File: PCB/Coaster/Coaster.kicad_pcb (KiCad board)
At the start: 2 copper layers, 202 x 100 mm, 84 parts, among them J1 Join, J2 Shelly, J3 USB-C, P1 TestPoint, P10 TestPoint, P11 TestPoint, P12 TestPoint, P13 TestPoint, P14 TestPoint, P15 TestPoint, P16 TestPoint, P17 TestPoint, P2 TestPoint, P5 TestPoint, P6 TestPoint, P7 TestPoint, P8 TestPoint, P9 TestPoint, T1 TestPoint, T10 TestPoint, T11 TestPoint, T12 TestPoint, T13 TestPoint, T14 TestPoint, T15 TestPoint, T16 TestPoint, T17 TestPoint, T2 TestPoint, T5 TestPoint, T6 TestPoint, T7 TestPoint, T8 TestPoint, T9 TestPoint, U1 ESP32-PICO-MINI-02, U2 LMR16006XDDCR, U3 QR

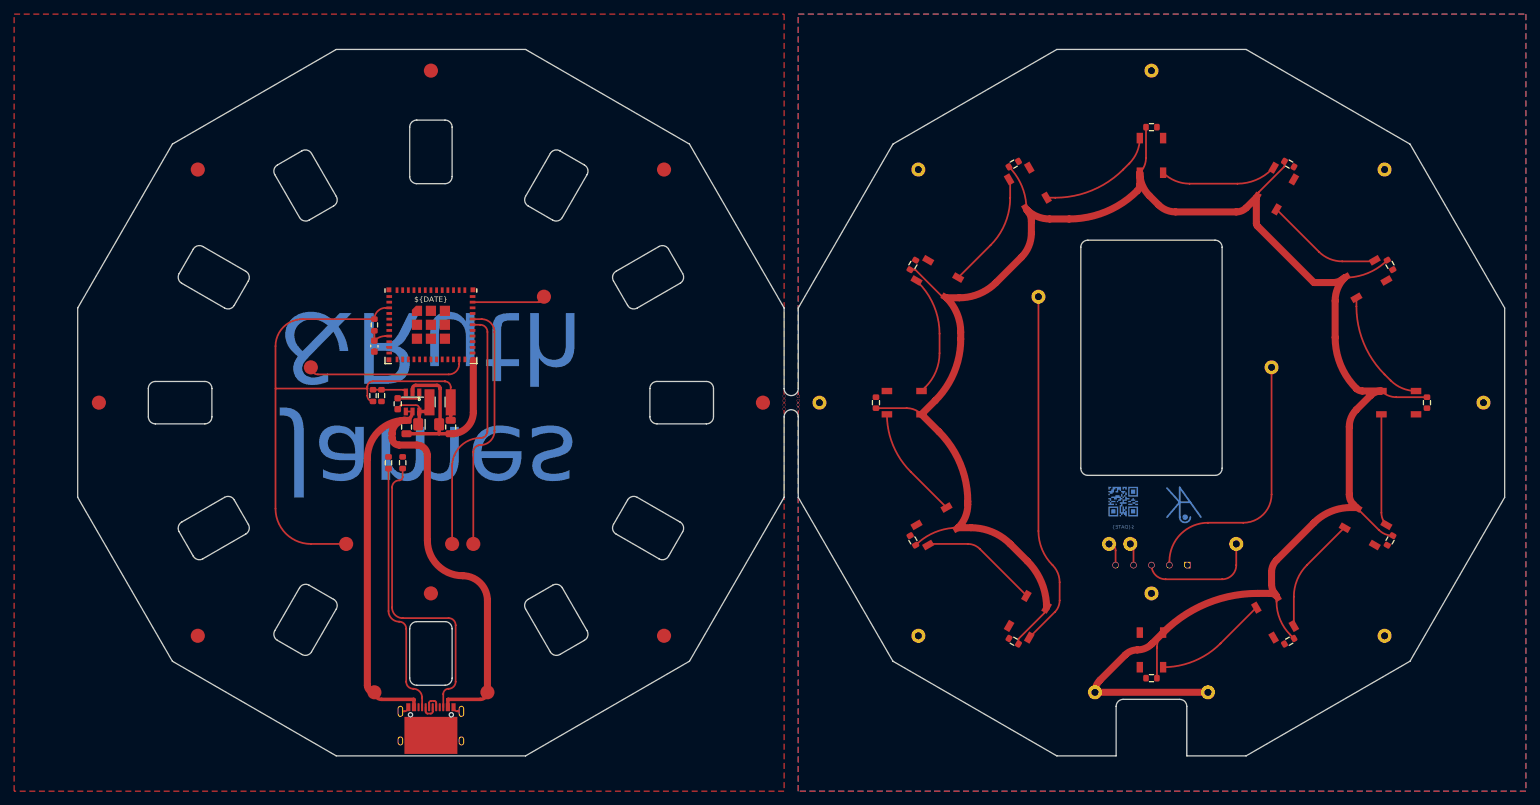
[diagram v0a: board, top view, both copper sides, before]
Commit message: Much tidying
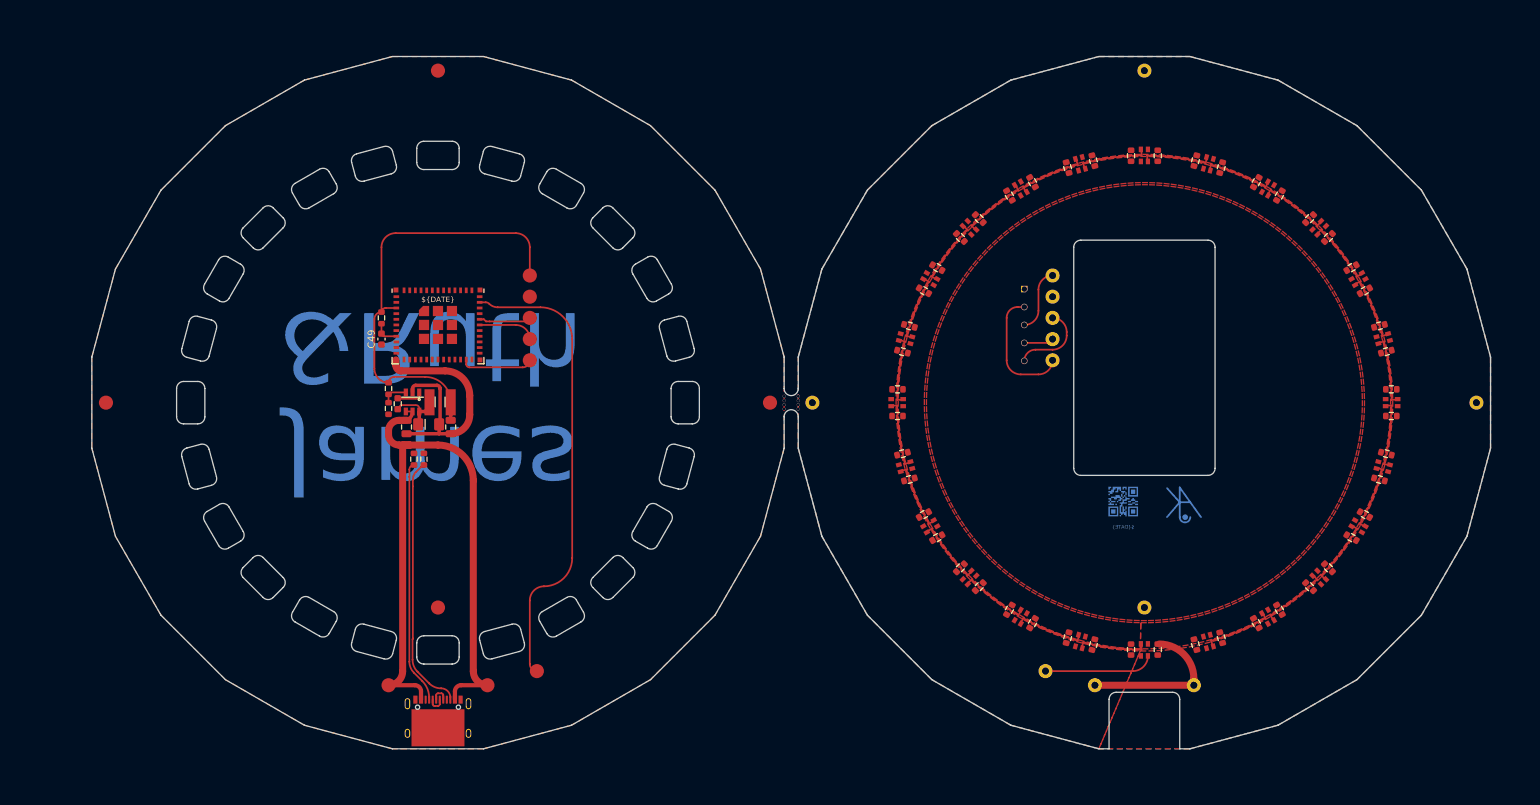
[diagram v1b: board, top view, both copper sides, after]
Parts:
- removed P13, P14, P15, P16, P17: TestPoint, RevK:PAD
- removed R6: 5K1, RevK:R_0603
- removed R7: 100k 1%, RevK:R_0603
- removed R8: 30k 1%, RevK:R_0603
- removed T13, T14, T15, T16, T17: TestPoint, RevK:PAD-LINK
- added C17: 10nF, RevK:C_0603, F.Cu at (229.3, 80.9)
- added C18: 10nF, RevK:C_0603, F.Cu at (233.3, 89.1)
- added C19: 10nF, RevK:C_0603, F.Cu at (234.9, 98.1)
- added C20: 10nF, RevK:C_0603, F.Cu at (234.2, 107.2)
- added C21: 10nF, RevK:C_0603, F.Cu at (231.2, 115.8)
- added C22: 10nF, RevK:C_0603, F.Cu at (226.1, 123.4)
- added C23: 10nF, RevK:C_0603, F.Cu at (219.1, 129.3)
- added C24: 10nF, RevK:C_0603, F.Cu at (210.9, 133.3)
- added C25: 10nF, RevK:C_0603, F.Cu at (198.1, 134.9)
- added C26: 10nF, RevK:C_0603, F.Cu at (189.1, 133.3)
- added C27: 10nF, RevK:C_0603, F.Cu at (180.9, 129.3)
- added C28: 10nF, RevK:C_0603, F.Cu at (173.9, 123.4)
- added C29: 10nF, RevK:C_0603, F.Cu at (168.8, 115.8)
- added C30: 10nF, RevK:C_0603, F.Cu at (165.8, 107.2)
- added C31: 10nF, RevK:C_0603, F.Cu at (165.1, 98.1)
- added C32: 10nF, RevK:C_0603, F.Cu at (166.7, 89.1)
- added C33: 10nF, RevK:C_0603, F.Cu at (170.7, 80.9)
- added C34: 10nF, RevK:C_0603, F.Cu at (176.6, 74.0)
- added C35: 10nF, RevK:C_0603, F.Cu at (184.2, 68.8)
- added C36: 10nF, RevK:C_0603, F.Cu at (192.8, 65.8)
- added C37: 10nF, RevK:C_0603, F.Cu at (201.9, 65.0)
- added C38: 10nF, RevK:C_0603, F.Cu at (210.9, 66.7)
- added C39: 10nF, RevK:C_0603, F.Cu at (219.1, 70.7)
- added C40: 10nF, RevK:C_0603, F.Cu at (226.1, 76.6)
- added C41: 10nF, RevK:C_0603, F.Cu at (231.2, 84.2)
- added C42: 10nF, RevK:C_0603, F.Cu at (234.2, 92.8)
- added C43: 10nF, RevK:C_0603, F.Cu at (234.9, 101.9)
- added C44: 10nF, RevK:C_0603, F.Cu at (233.3, 110.9)
- added C45: 10nF, RevK:C_0603, F.Cu at (229.3, 119.1)
- added C46: 10nF, RevK:C_0603, F.Cu at (223.4, 126.0)
- added C47: 10nF, RevK:C_0603, F.Cu at (215.8, 131.2)
- added C48: 10nF, RevK:C_0603, F.Cu at (207.2, 134.2)
- added C49: 10nF, Capacitor_SMD:C_0603_1608Metric, F.Cu at (92.0, 91.0)
- added C50: 100nF, RevK:C_0603_, F.Cu at (94.3, 100.2)
- added C51: 2.2uF, RevK:C_0805_, F.Cu at (95.5, 103.5)
- added C52: 10uF, RevK:C_0805_, F.Cu at (101.8, 103.5)
- added D13: WS2818B, RevK:SMD2020, F.Cu at (200.0, 65.0)
- added D15: WS2818B, RevK:SMD2020, F.Cu at (217.5, 69.7)
- added D16: WS2818B, RevK:SMD2020, F.Cu at (224.8, 75.2)
- added D17: WS2818B, RevK:SMD2020, F.Cu at (230.3, 82.5)
- added D18: WS2818B, RevK:SMD2020, F.Cu at (233.8, 90.9)
- added D19: WS2818B, RevK:SMD2020, F.Cu at (235.0, 100.0)
- added D20: WS2818B, RevK:SMD2020, F.Cu at (233.8, 109.1)
- added D21: WS2818B, RevK:SMD2020, F.Cu at (230.3, 117.5)
- added D22: WS2818B, RevK:SMD2020, F.Cu at (224.8, 124.8)
- added D23: WS2818B, RevK:SMD2020, F.Cu at (217.5, 130.3)
- added D24: WS2818B, RevK:SMD2020, F.Cu at (209.1, 133.8)
- added D25: Schottky, RevK:D_1206_, F.Cu at (98.7, 103.1)
- added H13: MountingHole, RevK:LEDHOLE, F.Cu at (100.0, 65.0)
- added H14: MountingHole, RevK:LEDHOLE, F.Cu at (109.1, 66.2)
- added H15: MountingHole, RevK:LEDHOLE, F.Cu at (117.5, 69.7)
- added H16: MountingHole, RevK:LEDHOLE, F.Cu at (124.8, 75.2)
- added H17: MountingHole, RevK:LEDHOLE, F.Cu at (130.3, 82.5)
- added H18: MountingHole, RevK:LEDHOLE, F.Cu at (133.8, 90.9)
- added H19: MountingHole, RevK:LEDHOLE, F.Cu at (135.0, 100.0)
- added H20: MountingHole, RevK:LEDHOLE, F.Cu at (133.8, 109.1)
- added H21: MountingHole, RevK:LEDHOLE, F.Cu at (130.3, 117.5)
- added H22: MountingHole, RevK:LEDHOLE, F.Cu at (124.8, 124.8)
- added H23: MountingHole, RevK:LEDHOLE, F.Cu at (117.5, 130.3)
- added H24: MountingHole, RevK:LEDHOLE, F.Cu at (109.1, 133.8)
- added P3: TestPoint, RevK:PAD, F.Cu at (113.0, 88.0)
- added P4: TestPoint, RevK:PAD, F.Cu at (113.0, 91.0)
- added R2: 5K1, RevK:R_0603, F.Cu at (96.6, 108.0)
- added R3: 5K1, RevK:R_0603, F.Cu at (98.0, 108.0)
- added R4: 100k 1%, RevK:R_0603, F.Cu at (93.0, 98.0)
- added T3: TestPoint, RevK:PAD-LINK, F.Cu at (187.0, 88.0)
- added T4: TestPoint, RevK:PAD-LINK, F.Cu at (187.0, 91.0)
- C13: value 100nF -> 10nF; footprint RevK:C_0603_ -> RevK:C_0603
- C14: value 2.2uF -> 10nF; footprint RevK:C_0805_ -> RevK:C_0603
- C15: value 10uF -> 10nF; footprint RevK:C_0805_ -> RevK:C_0603
- C16: footprint Capacitor_SMD:C_0603_1608Metric -> RevK:C_0603
- D1, D10, D11, D12, D2, D3, D4, D5, D6, D7, D8, D9: footprint RevK:SMD5050 -> RevK:SMD2020
- D14: value Schottky -> WS2818B; footprint RevK:D_1206_ -> RevK:SMD2020
- J1: value Join -> USB-C; footprint RevK:PCB-Join -> RevK:USC16-TR
- J3: value USB-C -> Join; footprint RevK:USC16-TR -> RevK:PCB-Join
- R5: value 5K1 -> 30k 1%
- moved C16 133.6 mm to (223.4, 74.0), turned to 45 degrees
- moved C15 119.2 mm to (215.8, 68.8), turned to 60 degrees
- moved C14 117.9 mm to (207.2, 65.8), turned to 75 degrees
- moved D14 116.4 mm to (209.1, 66.2), turned to 75 degrees
- moved C13 109.6 mm to (198.1, 65.0), turned to 90 degrees
- moved P7 86.3 mm to (114.0, 138.0)
- moved T7 86.3 mm to (186.0, 138.0)
- moved C5 74.8 mm to (170.7, 119.1), turned to -150 degrees
- moved P8 74.0 mm to (100.0, 53.0)
- moved T8 74.0 mm to (200.0, 53.0)
- moved D5 70.9 mm to (169.7, 117.5), turned to -150 degrees
- moved C6 69.9 mm to (166.7, 110.9), turned to -165 degrees
- moved H5 69.1 mm to (69.7, 117.5), turned to 120 degrees
- moved C4 68.5 mm to (176.6, 126.0), turned to -135 degrees
- moved J3 68.4 mm to (150.0, 100.0)
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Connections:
- C16 pad 1: GND -> VCC
- C16 pad 2: Net-(C16-Pad2) -> GND2
- D1 pad 2: unconnected-(D1-Pad2) -> Net-(D1-Pad2)
- D1 pad 4: Net-(D1-Pad4) -> LED
- D11 pad 2: Net-(D10-Pad4) -> Net-(D11-Pad2)
- D11 pad 4: Net-(D11-Pad4) -> Net-(D10-Pad2)
- D12 pad 2: Net-(D11-Pad4) -> Net-(D12-Pad2)
- D12 pad 4: LED -> Net-(D11-Pad2)
- D2 pad 2: Net-(D1-Pad4) -> Net-(D2-Pad2)
- D2 pad 4: Net-(D2-Pad4) -> Net-(D1-Pad2)
- D3 pad 2: Net-(D2-Pad4) -> Net-(D3-Pad2)
- D3 pad 4: Net-(D3-Pad4) -> Net-(D2-Pad2)
- D4 pad 2: Net-(D3-Pad4) -> Net-(D4-Pad2)
- D4 pad 4: Net-(D4-Pad4) -> Net-(D3-Pad2)
- D5 pad 2: Net-(D4-Pad4) -> Net-(D5-Pad2)
- D5 pad 4: Net-(D5-Pad4) -> Net-(D4-Pad2)
- D6 pad 2: Net-(D5-Pad4) -> Net-(D6-Pad2)
- D6 pad 4: Net-(D6-Pad4) -> Net-(D5-Pad2)
- D7 pad 2: Net-(D6-Pad4) -> Net-(D7-Pad2)
- D7 pad 4: Net-(D7-Pad4) -> Net-(D6-Pad2)
- D8 pad 2: Net-(D7-Pad4) -> Net-(D8-Pad2)
- D8 pad 4: Net-(D8-Pad4) -> Net-(D7-Pad2)
- D9 pad 2: Net-(D8-Pad4) -> Net-(D10-Pad4)
- D9 pad 4: Net-(D10-Pad2) -> Net-(D8-Pad2)
- P10 pad 1: Net-(P10-Pad1) -> GND
- P11 pad 1: +3V3 -> GND
- P12 pad 1: Net-(P12-Pad1) -> GND
- P5 pad 1: GND -> +3V3
- P6 pad 1: GND -> Net-(P6-Pad1)
- P7 pad 1: GND -> Net-(P7-Pad1)
- P9 pad 1: Net-(P9-Pad1) -> GND
- R1 pad 2: Net-(C16-Pad2) -> Net-(C49-Pad2)
- R5 pad 1: Net-(J3-PadB5) -> GND
- R5 pad 2: GND -> Net-(R4-Pad2)
- T10 pad 1: I -> GND2
- T11 pad 1: +3.3VA -> GND2
- T12 pad 1: GPIO0 -> GND2
- T5 pad 1: GND2 -> +3.3VA
- T6 pad 1: GND2 -> GPIO0
- T7 pad 1: GND2 -> LED
- T9 pad 1: O -> GND2
- U1 pad 23: Net-(P12-Pad1) -> Net-(P6-Pad1)
- U1 pad 30: Net-(P10-Pad1) -> Net-(P4-Pad1)
- U1 pad 31: Net-(P9-Pad1) -> Net-(P3-Pad1)
- U1 pad 34: Net-(P13-Pad1) -> Net-(P7-Pad1)
- U1 pad 8: Net-(C16-Pad2) -> Net-(C49-Pad2)
- U2 pad 3: Net-(R7-Pad2) -> Net-(R4-Pad2)
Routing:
- net VCC: track 321.3 -> 22.4 mm
- net Net-(P7-Pad1): track 0.00 -> 66.4 mm
- net Net-(J3-PadB5): track 43.3 -> 0.00 mm
- net Net-(J3-PadA5): track 36.3 -> 0.00 mm
- net Net-(J1-PadB5): track 0.00 -> 36.3 mm
- net Net-(P9-Pad1): track 35.7 -> 0.00 mm
- net Net-(P10-Pad1): track 35.3 -> 0.00 mm
- net LED: track 50.7 -> 15.6 mm
- net Net-(J1-PadA5): track 0.00 -> 34.2 mm
- net +3V3: track 84.9 -> 61.4 mm
- net Net-(P12-Pad1): track 23.0 -> 0.00 mm
- net GPIO0: track 38.0 -> 17.9 mm
- net Net-(D7-Pad4): track 17.0 -> 0.00 mm
- net Net-(D4-Pad4): track 17.0 -> 0.00 mm
- net Net-(D2-Pad4): track 16.5 -> 0.00 mm
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- added copper zone on F.Cu, net VCC
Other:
- board size 202 x 100 mm -> 198 x 98 mm
